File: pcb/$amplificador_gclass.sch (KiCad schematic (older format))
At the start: 49 parts, among them CON1 AUDIO_IN, P1 CONN_01X01, P10 CONN_01X01, P12 OUT, P13 CONN_01X01, P2 CONN_01X01, P3 CONN_01X01, P4 CONN_01X01, P5 +VA_GND, P6 +VB_GND, P7 -VA_GND, P8 -VB_GND, P9 CONN_01X01, Q1 MPSA56_PNP_EBC, Q10 MPSA06_NPN_EBC, Q11 MPSA56_PNP_EBC, Q12 MPSA06_NPN_EBC, Q2 MPSA56_PNP_EBC, Q3 MPSA06_NPN_EBC, Q4 MPSA56_PNP_EBC, Q5 MPSA06_NPN_EBC, Q6 MPSA56_PNP_EBC, Q7 MPSA56_PNP_EBC, Q8 MPSA56_PNP_EBC, Q9 MPSA56_PNP_EBC

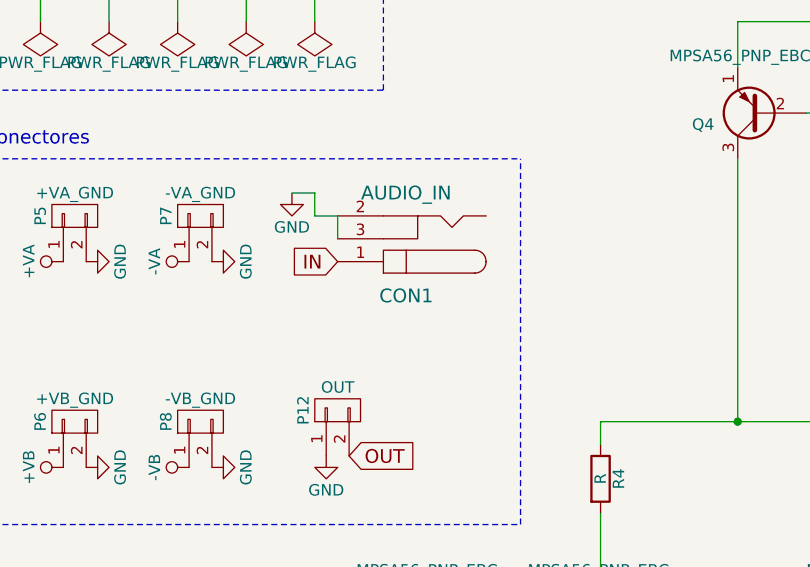
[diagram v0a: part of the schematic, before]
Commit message: pcb terminado
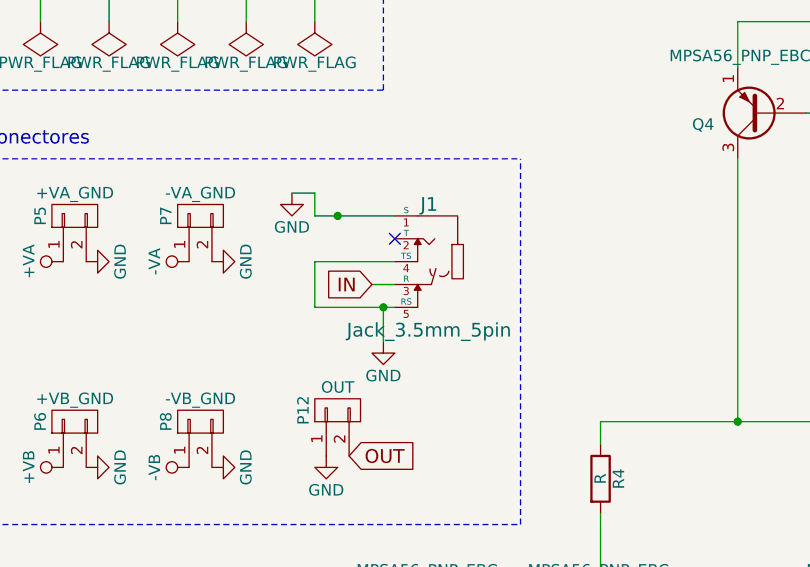
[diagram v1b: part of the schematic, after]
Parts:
- removed CON1: AUDIO_IN, Connect:BARREL_JACK, symbol BARREL_JACK
- added J1: Jack_3.5mm_5pin, pcb:jack_puto, symbol Jack_3.5mm_5pin
- P1, P2, P3, P4: footprint Socket_Strips:Socket_Strip_Straight_1x02 -> Pin_Headers:Pin_Header_Straight_1x01
- P10, P9: footprint pcb:bornera_grande -> Pin_Headers:Pin_Header_Straight_1x01
- P12: footprint pcb:bornera_grande -> Pin_Headers:Pin_Header_Straight_1x02
- P6: footprint Pin_Headers:Pin_Header_Straight_1x01 -> Pin_Headers:Pin_Header_Straight_1x02
- P7, P8: footprint pcb:bornera_chica -> Pin_Headers:Pin_Header_Straight_1x02
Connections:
- net GND: now also J1.1 (S), J1.4 (TS), J1.5 (RS)
- net IN: now also J1.3 (R)
- no-connect marks 0 -> 1
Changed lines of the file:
@@
 LIBS:contrib
 LIBS:valves
+LIBS:w_connectors
 LIBS:amplificador_gclass-cache
 EELAYER 25 0
@@
 F 0 "P8" H 2000 3400 50  0000 C CNN
 F 1 "-VB_GND" V 2100 3250 50  0000 C CNN
-F 2 "pcb:bornera_chica" H 2000 3250 60  0001 C CNN
+F 2 "Pin_Headers:Pin_Header_Straight_1x02" H 2000 3250 60  0001 C CNN
 F 3 "" H 2000 3250 60  0000 C CNN
 	1    2000 3250
@@
 F 0 "P6" H 1450 3400 50  0000 C CNN
 F 1 "+VB_GND" V 1550 3250 50  0000 C CNN
-F 2 "Pin_Headers:Pin_Header_Straight_1x01" H 1450 3250 60  0001 C CNN
+F 2 "Pin_Headers:Pin_Header_Straight_1x02" H 1450 3250 60  0001 C CNN
 F 3 "" H 1450 3250 60  0000 C CNN
 	1    1450 3250
@@
 F 0 "P7" H 2000 2500 50  0000 C CNN
 F 1 "-VA_GND" V 2100 2350 50  0000 C CNN
-F 2 "pcb:bornera_chica" H 2000 2350 60  0001 C CNN
+F 2 "Pin_Headers:Pin_Header_Straight_1x02" H 2000 2350 60  0001 C CNN
 F 3 "" H 2000 2350 60  0000 C CNN
 	1    2000 2350
@@
 Wire Notes Line
 	2800 1800 2800 1000
-Text GLabel 2600 2550 0    60   Input ~ 0
+Text GLabel 2750 2650 0    60   Input ~ 0
 IN
 $Comp
@@
 F 0 "P12" H 2600 3350 50  0000 C CNN
 F 1 "OUT" V 2700 3200 50  0000 C CNN
-F 2 "pcb:bornera_grande" H 2600 3200 60  0001 C CNN
+F 2 "Pin_Headers:Pin_Header_Straight_1x02" H 2600 3200 60  0001 C CNN
 F 3 "" H 2600 3200 60  0000 C CNN
 	1    2600 3200
 	0    -1   -1   0
 $EndComp
-$Comp
-L BARREL_JACK CON1
-U 1 1 556D4923
-P 2900 2450
-F 0 "CON1" H 2900 2700 60  0000 C CNN
-F 1 "AUDIO_IN" H 2900 2250 60  0000 C CNN
-F 2 "Connect:BARREL_JACK" H 2900 2450 60  0001 C CNN
-F 3 "" H 2900 2450 60  0000 C CNN
-	1    2900 2450
-	-1   0    0    1
-$EndComp
 Wire Wire Line
 	2400 2250 2500 2250
@@
 	2500 2250 2500 2350
 Wire Wire Line
-	2500 2350 2600 2350
-Wire Wire Line
-	2600 2350 2600 2450
+	2500 2350 2850 2350
 Wire Notes Line
 	3400 3700 3400 2100
@@
 F 0 "P1" H 1250 6200 50  0000 C CNN
 F 1 "CONN_01X01" H 1250 5950 50  0000 C CNN
-F 2 "Socket_Strips:Socket_Strip_Straight_1x02" H 1250 6100 60  0001 C CNN
+F 2 "Pin_Headers:Pin_Header_Straight_1x01" H 1250 6100 60  0001 C CNN
 F 3 "" H 1250 6100 60  0000 C CNN
 	1    1250 6100
@@
 F 0 "P2" H 1250 6600 50  0000 C CNN
 F 1 "CONN_01X01" H 1250 6350 50  0000 C CNN
-F 2 "Socket_Strips:Socket_Strip_Straight_1x02" H 1250 6500 60  0001 C CNN
+F 2 "Pin_Headers:Pin_Header_Straight_1x01" H 1250 6500 60  0001 C CNN
 F 3 "" H 1250 6500 60  0000 C CNN
 	1    1250 6500
@@
 F 0 "P3" H 1250 7050 50  0000 C CNN
 F 1 "CONN_01X01" H 1250 6800 50  0000 C CNN
-F 2 "Socket_Strips:Socket_Strip_Straight_1x02" H 1250 6950 60  0001 C CNN
+F 2 "Pin_Headers:Pin_Header_Straight_1x01" H 1250 6950 60  0001 C CNN
 F 3 "" H 1250 6950 60  0000 C CNN
 	1    1250 6950
@@
 F 0 "P4" H 1250 7500 50  0000 C CNN
 F 1 "CONN_01X01" H 1250 7250 50  0000 C CNN
-F 2 "Socket_Strips:Socket_Strip_Straight_1x02" H 1250 7400 60  0001 C CNN
+F 2 "Pin_Headers:Pin_Header_Straight_1x01" H 1250 7400 60  0001 C CNN
 F 3 "" H 1250 7400 60  0000 C CNN
 	1    1250 7400
@@
 F 0 "P10" H 2100 6900 50  0000 C CNN
 F 1 "CONN_01X01" H 2100 6650 50  0000 C CNN
-F 2 "pcb:bornera_grande" H 2100 6800 60  0001 C CNN
+F 2 "Pin_Headers:Pin_Header_Straight_1x01" H 2100 6800 60  0001 C CNN
 F 3 "" H 2100 6800 60  0000 C CNN
 	1    2100 6800
@@
 $EndComp
 $Comp
-L GND #PWR036
+L GND #PWR035
 U 1 1 5577E81F
 P 2400 6850
-F 0 "#PWR036" H 2400 6600 50  0001 C CNN
+F 0 "#PWR035" H 2400 6600 50  0001 C CNN
 F 1 "GND" H 2400 6700 50  0000 C CNN
 F 2 "" H 2400 6850 60  0000 C CNN
@@
 F 0 "P9" H 2100 6200 50  0000 C CNN
 F 1 "CONN_01X01" H 2100 5950 50  0000 C CNN
-F 2 "pcb:bornera_grande" H 2100 6100 60  0001 C CNN
+F 2 "Pin_Headers:Pin_Header_Straight_1x01" H 2100 6100 60  0001 C CNN
 F 3 "" H 2100 6100 60  0000 C CNN
 	1    2100 6100
@@
 $EndComp
 $Comp
-L GND #PWR037
+L GND #PWR036
 U 1 1 5579C52B
 P 2400 6150
-F 0 "#PWR037" H 2400 5900 50  0001 C CNN
+F 0 "#PWR036" H 2400 5900 50  0001 C CNN
 F 1 "GND" H 2400 6000 50  0000 C CNN
 F 2 "" H 2400 6150 60  0000 C CNN
@@
 Wire Wire Line
 	2400 6100 2400 6150
+$Comp
+L Jack_3.5mm_5pin J1
+U 1 1 557AAF8F
+P 3000 2550
+F 0 "J1" H 3000 2800 60  0000 C CNN
+F 1 "Jack_3.5mm_5pin" H 3000 2250 60  0000 C CNN
+F 2 "pcb:jack_puto" H 3000 2600 60  0001 C CNN
+F 3 "" H 3000 2600 60  0000 C CNN
+	1    3000 2550
+	1    0    0    -1
+$EndComp
+Connection ~ 2600 2350
+Wire Wire Line
+	2750 2650 2850 2650
+NoConn ~ 2850 2450
+$Comp
+L GND #PWR037
+U 1 1 557AC041
+P 2800 2900
+F 0 "#PWR037" H 2800 2650 50  0001 C CNN
+F 1 "GND" H 2800 2750 50  0000 C CNN
+F 2 "" H 2800 2900 60  0000 C CNN
+F 3 "" H 2800 2900 60  0000 C CNN
+	1    2800 2900
+	1    0    0    -1
+$EndComp
+Wire Wire Line
+	2800 2900 2800 2750
+Wire Wire Line
+	2500 2750 2850 2750
+Wire Wire Line
+	2850 2550 2500 2550
+Wire Wire Line
+	2500 2550 2500 2750
+Connection ~ 2800 2750
 $EndSCHEMATC
